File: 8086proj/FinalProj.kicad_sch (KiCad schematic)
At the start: 0 parts

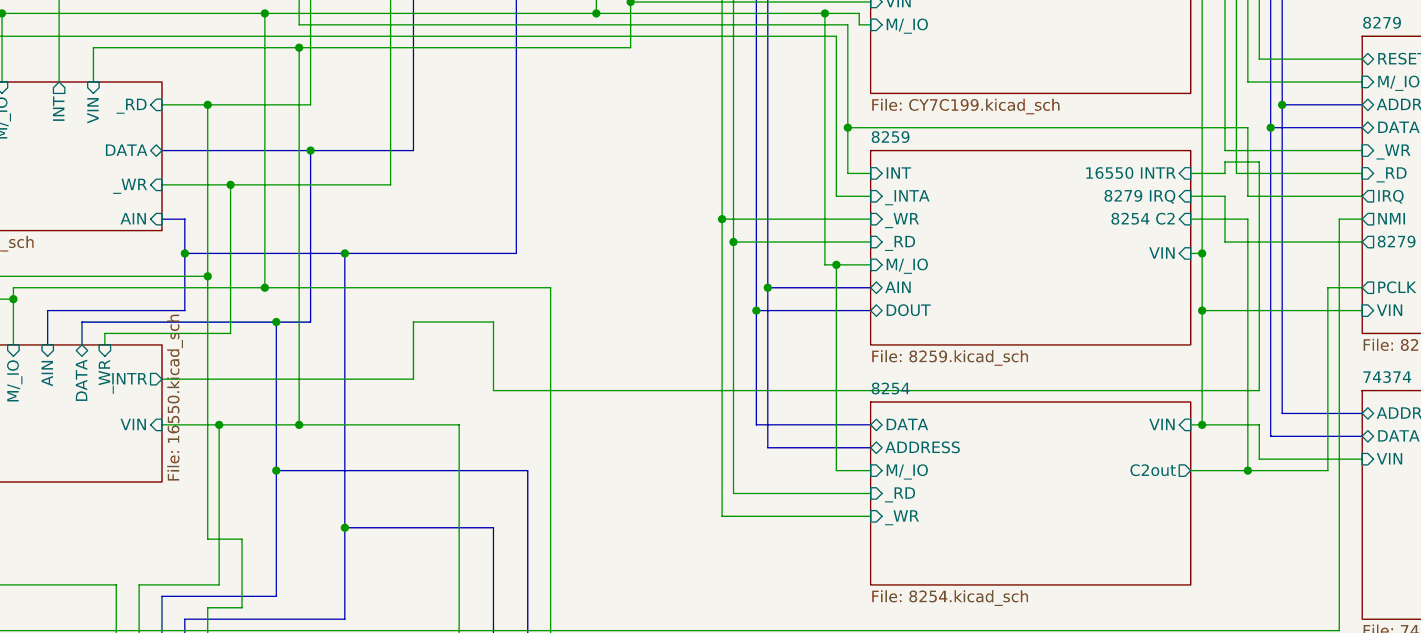
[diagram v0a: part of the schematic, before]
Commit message: pcb edit
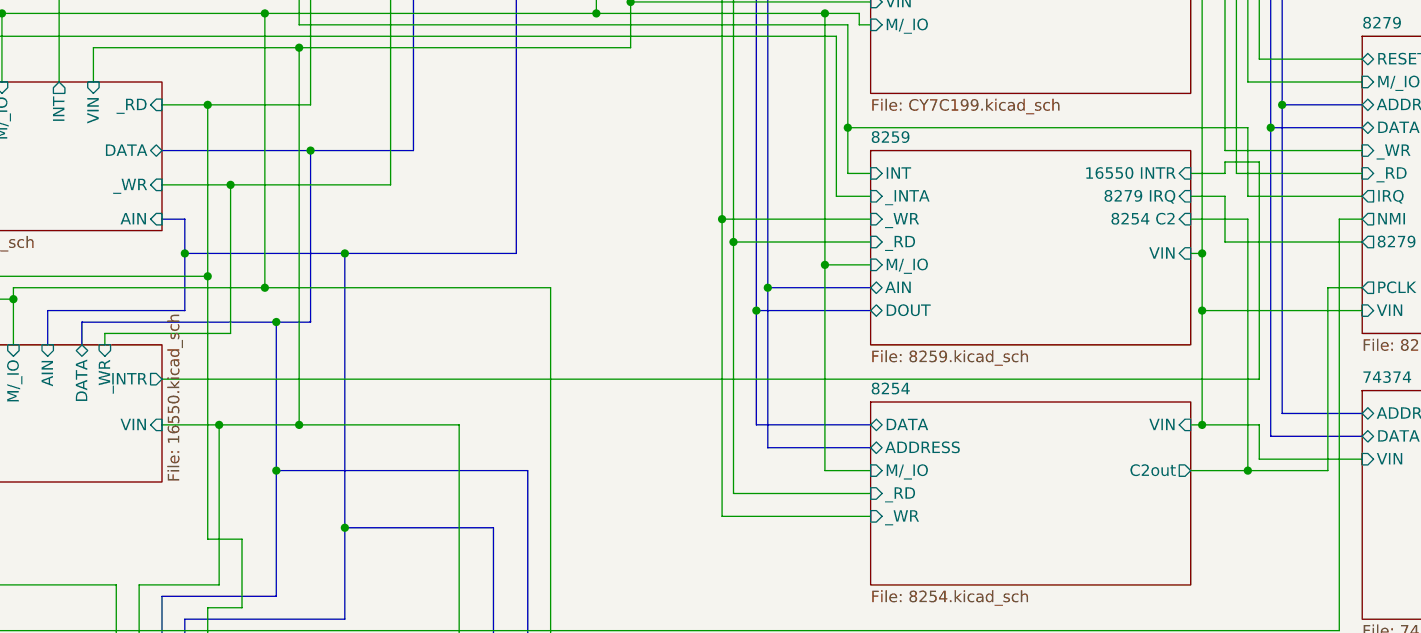
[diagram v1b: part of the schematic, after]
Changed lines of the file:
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@@
   (junction (at 142.24 120.65) (diameter 0) (color 0 0 0 0)
   )
+  (junction (at 152.4 123.19) (diameter 0) (color 0 0 0 0)
+  )
   (junction (at 72.39 22.86) (diameter 0) (color 0 0 0 0)
   )
@@
   (junction (at 144.78 86.36) (diameter 0) (color 0 0 0 0)
   )
-  (junction (at 153.67 123.19) (diameter 0) (color 0 0 0 0)
-  )
   (junction (at 62.23 127) (diameter 0) (color 0 0 0 0)
   )
@@
     (stroke (width 0) (type default) (color 0 0 0 0))
   )
-  (wire (pts (xy 78.74 135.89) (xy 106.68 135.89))
-    (stroke (width 0) (type default) (color 0 0 0 0))
-  )
   (wire (pts (xy 53.34 97.79) (xy 53.34 102.87))
     (stroke (width 0) (type default) (color 0 0 0 0))
@@
     (stroke (width 0) (type default) (color 0 0 0 0))
   )
-  (wire (pts (xy 115.57 137.16) (xy 200.66 137.16))
+  (wire (pts (xy 78.74 135.89) (xy 200.66 135.89))
     (stroke (width 0) (type default) (color 0 0 0 0))
   )
@@
     (stroke (width 0) (type default) (color 0 0 0 0))
   )
-  (wire (pts (xy 153.67 146.05) (xy 157.48 146.05))
+  (wire (pts (xy 152.4 146.05) (xy 157.48 146.05))
     (stroke (width 0) (type default) (color 0 0 0 0))
   )
@@
     (stroke (width 0) (type default) (color 0 0 0 0))
   )
-  (wire (pts (xy 106.68 129.54) (xy 115.57 129.54))
-    (stroke (width 0) (type default) (color 0 0 0 0))
-  )
   (wire (pts (xy 72.39 130.81) (xy 72.39 132.08))
     (stroke (width 0) (type default) (color 0 0 0 0))
@@
     (stroke (width 0) (type default) (color 0 0 0 0))
   )
-  (wire (pts (xy 153.67 123.19) (xy 153.67 146.05))
+  (wire (pts (xy 152.4 123.19) (xy 152.4 146.05))
     (stroke (width 0) (type default) (color 0 0 0 0))
   )
@@
     (stroke (width 0) (type default) (color 0 0 0 0))
   )
-  (wire (pts (xy 200.66 137.16) (xy 200.66 111.76))
+  (wire (pts (xy 200.66 135.89) (xy 200.66 111.76))
     (stroke (width 0) (type default) (color 0 0 0 0))
   )
@@
     (stroke (width 0) (type default) (color 0 0 0 0))
   )
-  (wire (pts (xy 106.68 135.89) (xy 106.68 129.54))
-    (stroke (width 0) (type default) (color 0 0 0 0))
-  )
   (wire (pts (xy 97.79 59.69) (xy 97.79 78.74))
     (stroke (width 0) (type default) (color 0 0 0 0))
@@
     (stroke (width 0) (type default) (color 0 0 0 0))
   )
-  (wire (pts (xy 153.67 123.19) (xy 157.48 123.19))
+  (wire (pts (xy 152.4 123.19) (xy 157.48 123.19))
     (stroke (width 0) (type default) (color 0 0 0 0))
   )
@@
     (stroke (width 0) (type default) (color 0 0 0 0))
   )
-  (wire (pts (xy 152.4 123.19) (xy 153.67 123.19))
-    (stroke (width 0) (type default) (color 0 0 0 0))
-  )
   (wire (pts (xy 83.82 105.41) (xy 83.82 124.46))
     (stroke (width 0) (type default) (color 0 0 0 0))
   )
-  (wire (pts (xy 115.57 129.54) (xy 115.57 137.16))
-    (stroke (width 0) (type default) (color 0 0 0 0))
-  )
